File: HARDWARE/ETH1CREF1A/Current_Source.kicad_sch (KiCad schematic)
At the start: 33 parts, among them U1002 LT5400-3, U1003 ADA4898-2, U1004 AD811JRZ, U1005 AQY211G2SX, U1006 AQY211G2SX, U1007 AQY211G2SX, U1008 AQY211G2SX, U1009 AQY211G2SX, U1010 AQY211G2SX, U601 DG419DY

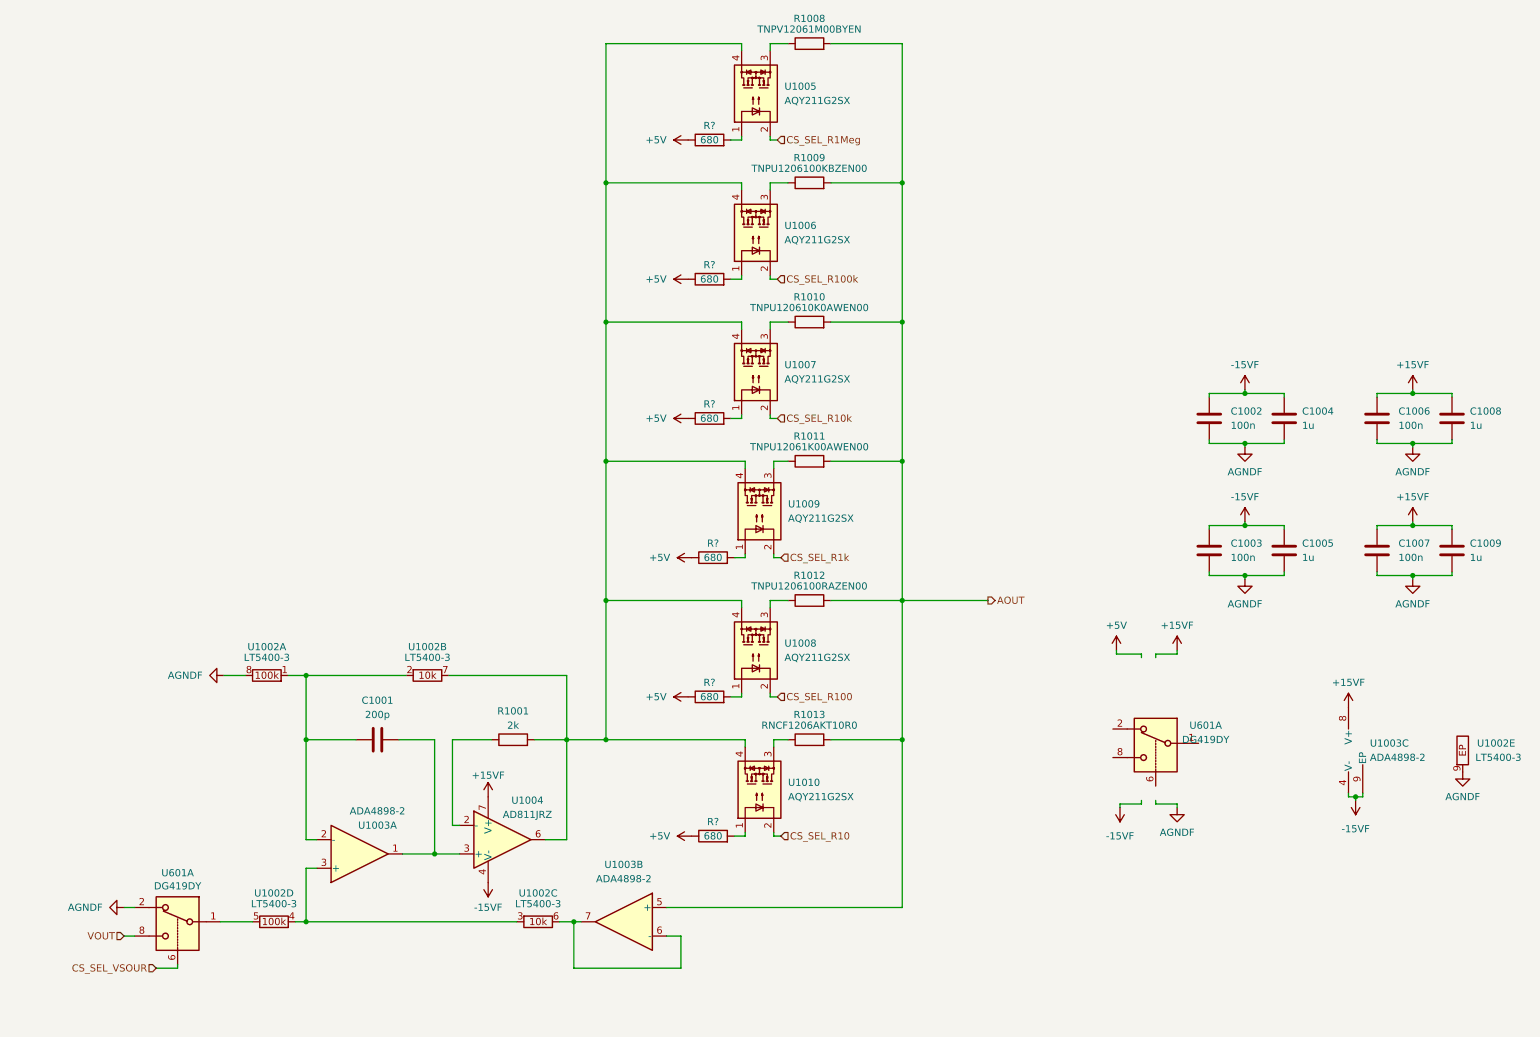
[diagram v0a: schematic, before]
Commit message: Hardware
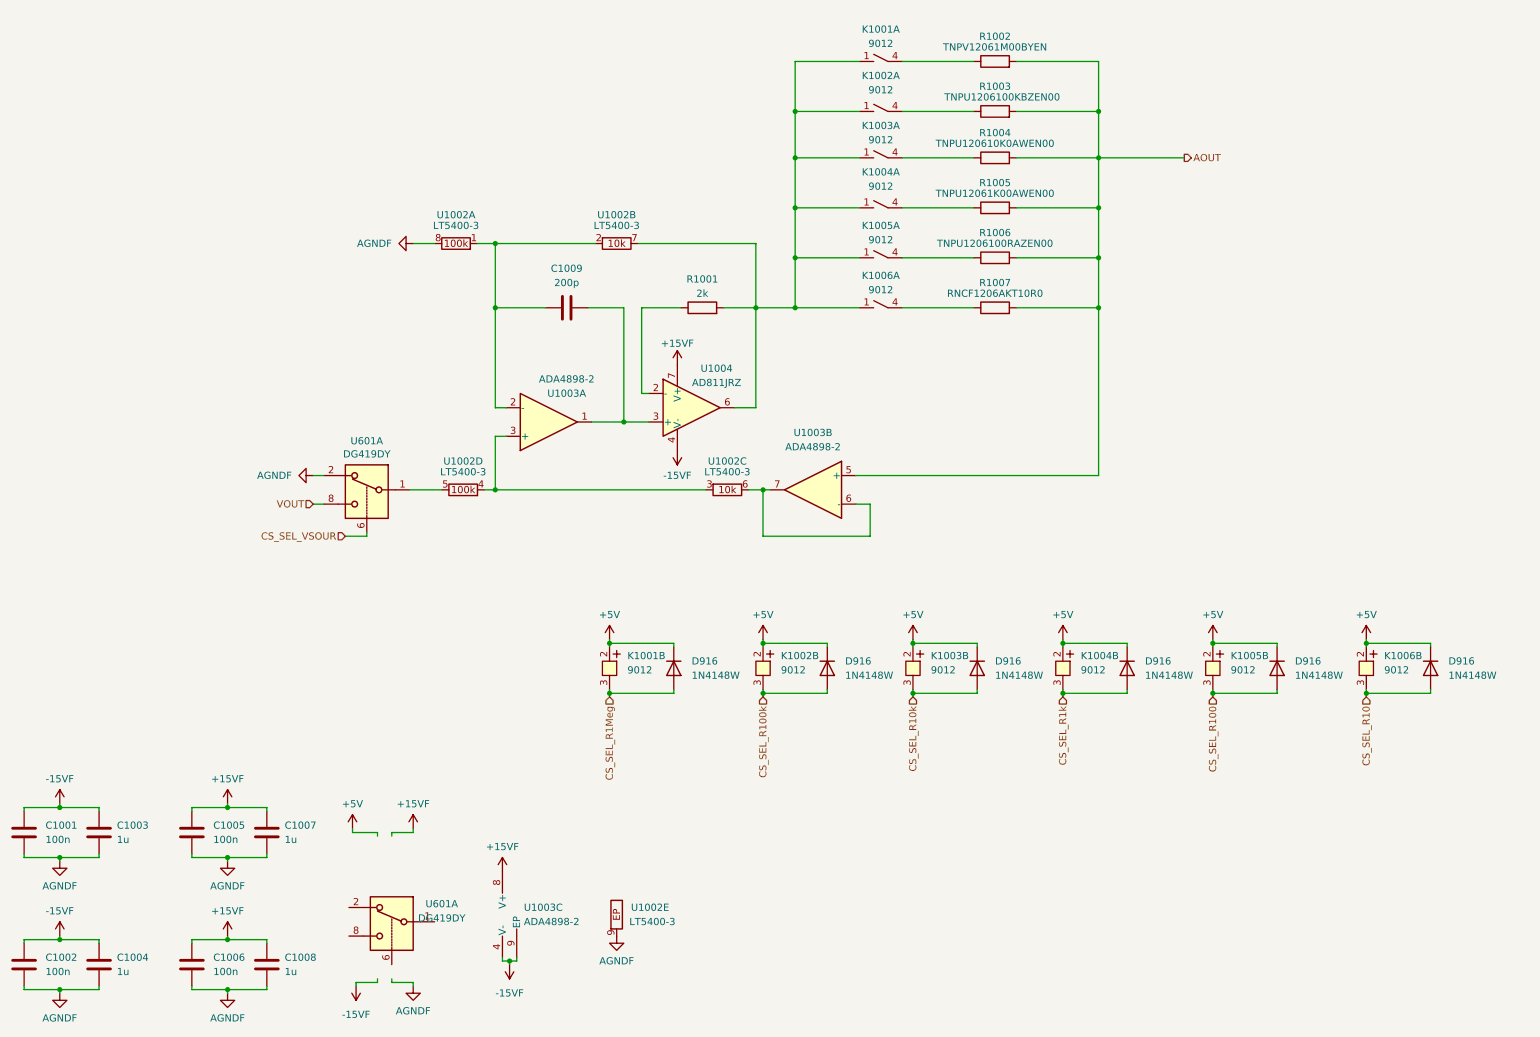
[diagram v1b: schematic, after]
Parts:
- removed R? (x6): 680, Resistor_SMD:R_0603_1608Metric_Pad0.98x0.95mm_HandSolder, symbol Device:R
- removed U1005, U1006, U1007, U1008, U1009, U1010: AQY211G2SX, ETH1CREF1A:AQY212GS, symbol ETH1CREF1A:AQY212GS
- added D916 (x6): 1N4148W, Diode_SMD:D_SOD-123, symbol Diode:1N4148W
- added K1001, K1002, K1003, K1004, K1005, K1006: 9012, ETH1CREF1A:9012, symbol ETH1CREF1A:9012
- renumbered C1002 to C1001, C1003 to C1002, C1004 to C1003, C1005 to C1004, C1006 to C1005, C1007 to C1006, C1008 to C1007, C1009 to C1008, C1001 to C1009, R1008 to R1002, R1009 to R1003, R1010 to R1004, R1011 to R1005, R1012 to R1006, R1013 to R1007
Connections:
- net +5V: now also D916.1 (K), D916.1 (K), D916.1 (K), D916.1 (K), D916.1 (K), D916.1 (K), K1001.2, K1002.2, K1003.2, K1004.2, K1005.2, K1006.2
- net CS_SEL_R10: now also D916.2 (A), K1006.3
- net CS_SEL_R100: now also D916.2 (A), K1005.3
- net CS_SEL_R100k: now also D916.2 (A), K1002.3
- net CS_SEL_R10k: now also D916.2 (A), K1003.3
- net CS_SEL_R1Meg: now also D916.2 (A), K1001.3
- net CS_SEL_R1k: now also D916.2 (A), K1004.3
- net at R1006.1: now also K1005.4
- net at R1001.2, U1002.7, U1004.6: now also K1001.1, K1002.1, K1003.1, K1004.1, K1005.1, K1006.1
- net at R1007.1: now also K1006.4
- net at R1005.1: now also K1004.4
- net at R1002.1: now also K1001.4
- net at R1003.1: now also K1002.4
- net at R1004.1: now also K1003.4
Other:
- moved on the sheet: C1001, C1002, C1003, C1004, C1005, C1006, C1007, C1008, C1009, R1001, R1002, R1003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
